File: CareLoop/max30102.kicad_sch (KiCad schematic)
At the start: 10 parts, among them U1 MCP1727-1802xMF, U2 MAX30102

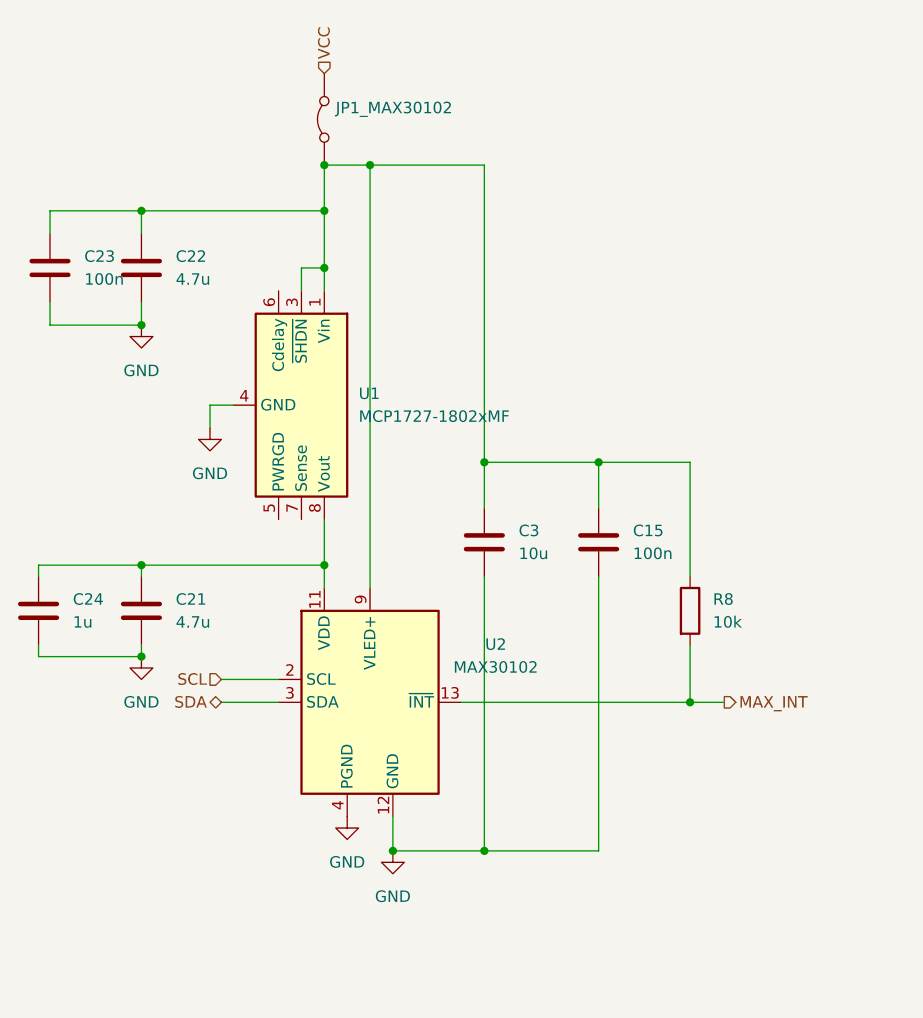
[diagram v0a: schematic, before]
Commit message: WP: update Schematics
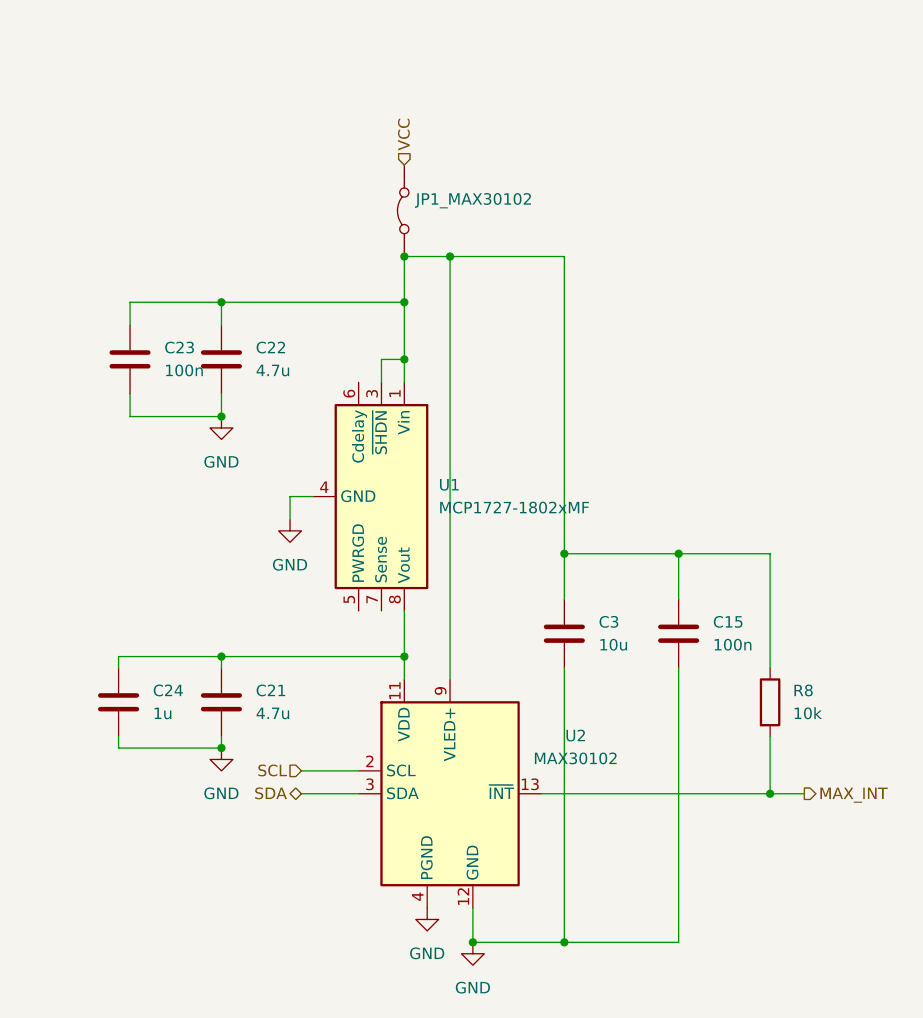
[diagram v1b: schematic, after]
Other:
- moved on the sheet: C15, C21, C22, C23, C24, C3, JP1_MAX30102, R8, U1, U2
